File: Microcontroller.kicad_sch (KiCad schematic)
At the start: 36 parts, among them IC201 ESP32-S3-WROOM-1-N4, SW201 NRST, SW202 USER, SW203 USER, SW204 USER, U201 STM32F405RGTx, Y201 16MHz|9p|10ppm

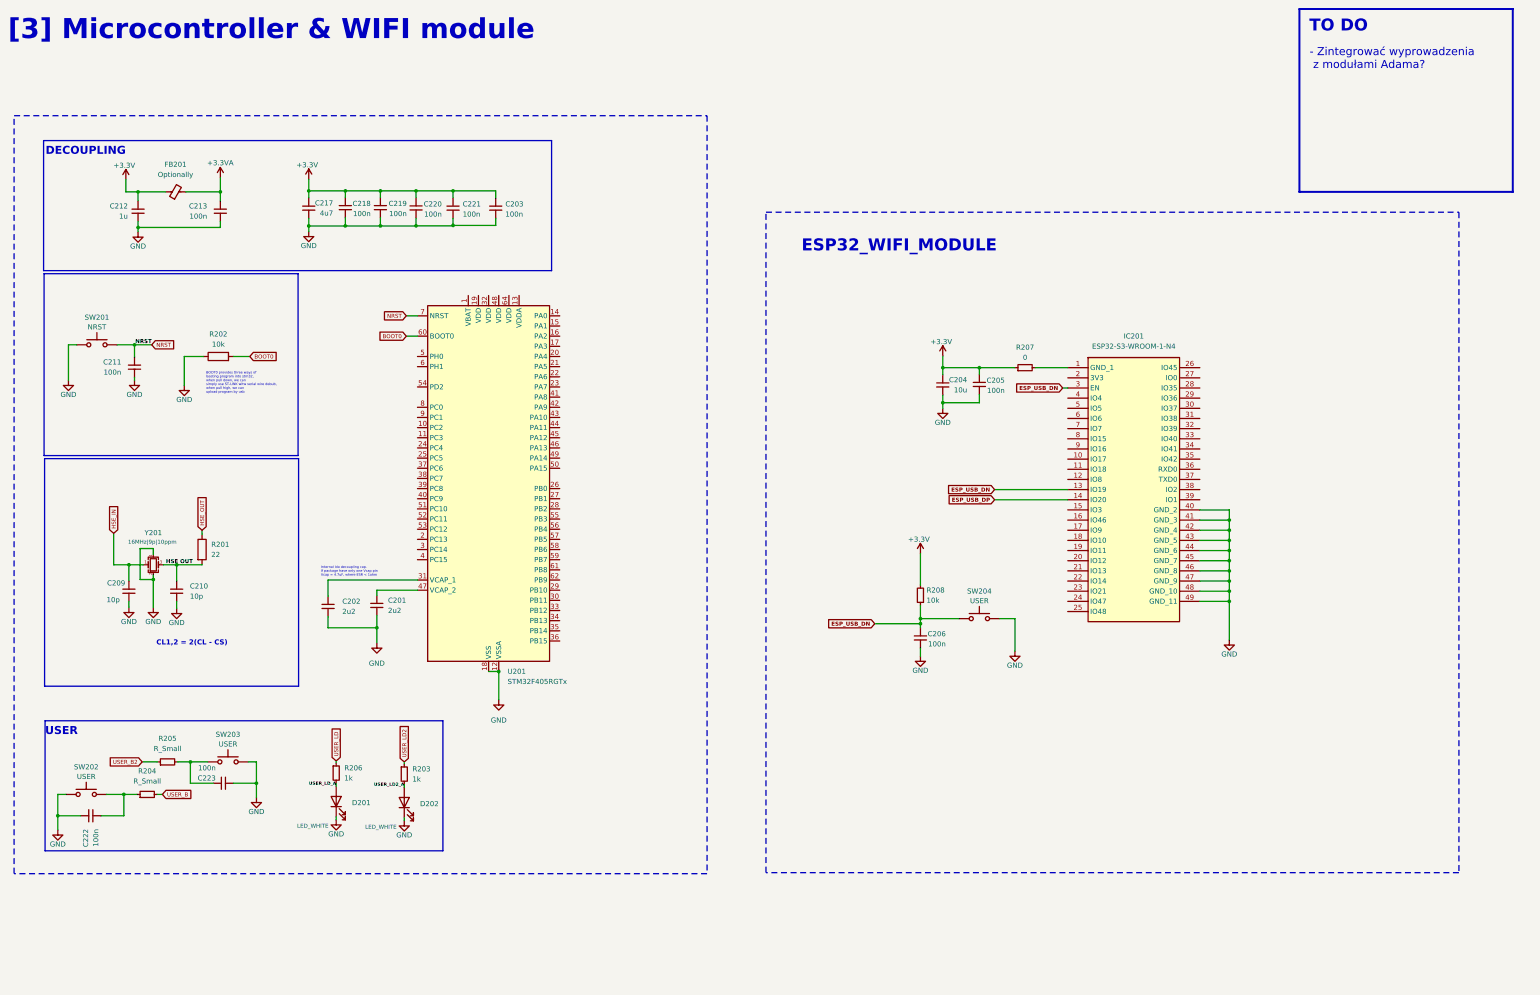
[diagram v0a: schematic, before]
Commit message: Dodaje wszystko nie chce mi sie z tym bawic
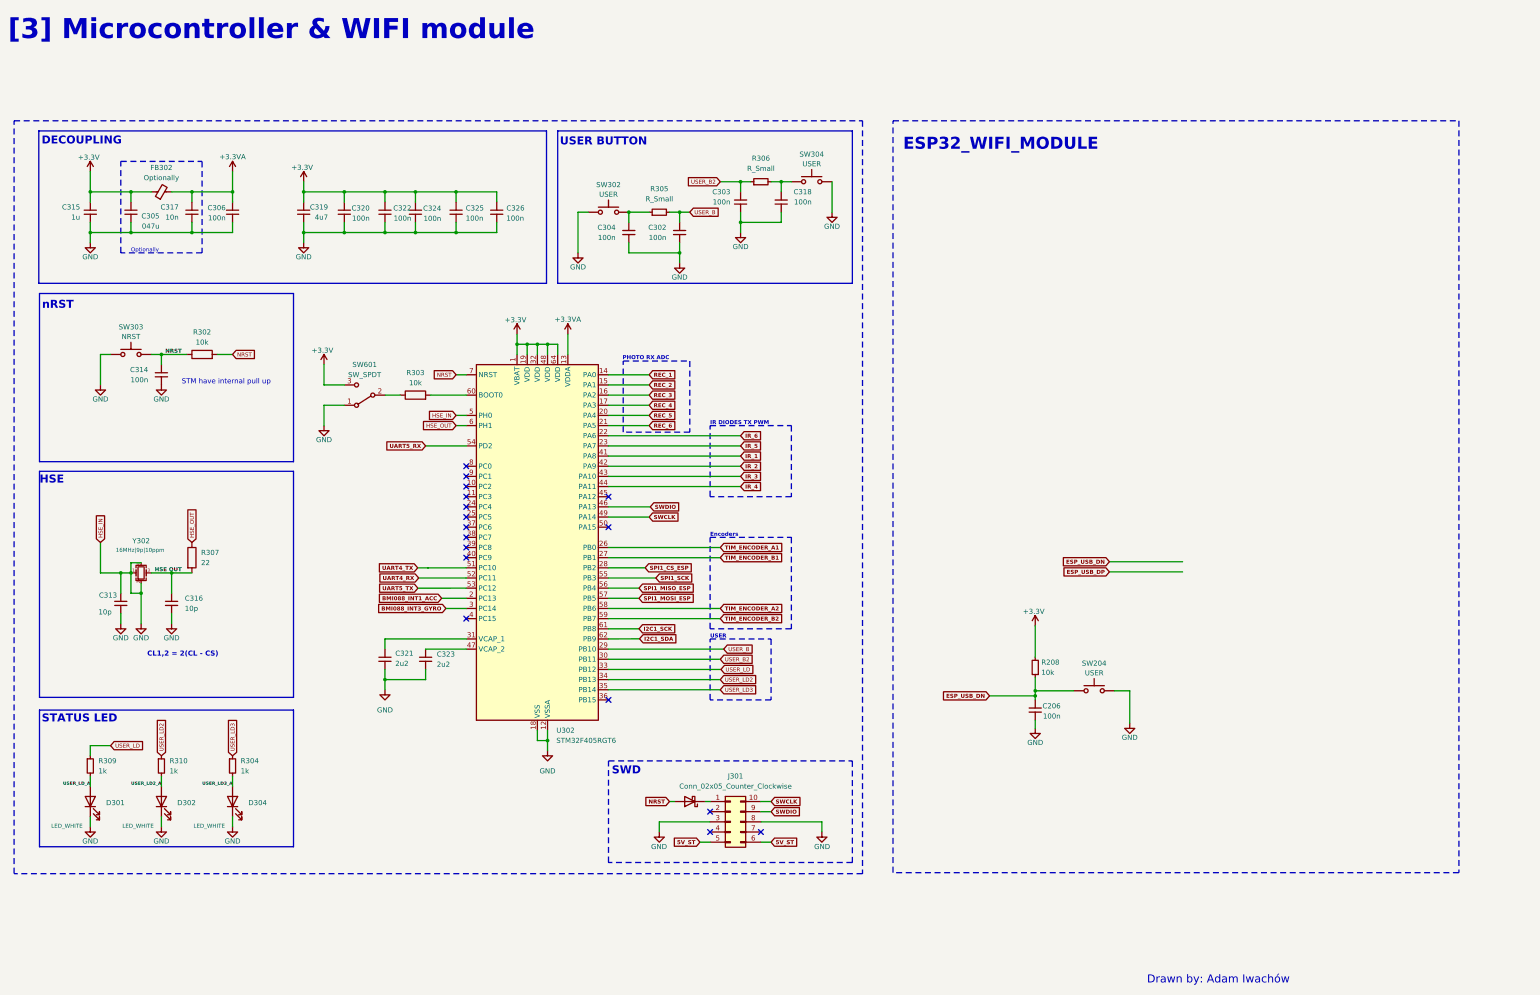
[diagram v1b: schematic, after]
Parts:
- removed C201, C202: 2u2, symbol Device:C_Small
- removed C203, C205, C211, C213, C218, C219, C220, C221, C222, C223: 100n, Capacitor_SMD:C_0402_1005Metric, symbol Device:C_Small
- removed C204: 10u, Capacitor_SMD:C_0603_1608Metric, symbol Device:C_Small
- removed C209, C210: 10p, Capacitor_SMD:C_0402_1005Metric, symbol Device:C_Small
- removed C212: 1u, Capacitor_SMD:C_0603_1608Metric, symbol Device:C_Small
- removed C217: 4u7, Capacitor_SMD:C_0603_1608Metric, symbol Device:C_Small
- removed D201, D202: LED_WHITE, Diode_SMD:D_0603_1608Metric, symbol Device:LED
- removed FB201: Optionally, symbol Device:FerriteBead_Small
- removed IC201: ESP32-S3-WROOM-1-N4, ESP32S3WROOM1N4, symbol SamacSys_Parts:ESP32-S3-WROOM-1-N4
- removed R201: 22, Resistor_SMD:R_0402_1005Metric, symbol Device:R
- removed R202: 10k, Resistor_SMD:R_0402_1005Metric, symbol Device:R
- removed R203, R206: 1k, Resistor_SMD:R_0603_1608Metric, symbol Device:R_Small
- removed R204, R205: R_Small, symbol Device:R_Small
- removed R207: 0, symbol Device:R_Small
- removed SW201: NRST, Button_Switch_SMD:SW_Push_1P1T_NO_6x6mm_H9.5mm, symbol Switch:SW_MEC_5G
- removed SW202, SW203: USER, Button_Switch_SMD:SW_Push_1P1T_NO_6x6mm_H9.5mm, symbol Switch:SW_MEC_5G
- removed U201: STM32F405RGTx, Package_QFP:LQFP-64_10x10mm_P0.5mm, symbol MCU_ST_STM32F4:STM32F405RGTx
- removed Y201: 16MHz|9p|10ppm, Crystal:Crystal_SMD_3225-4Pin_3.2x2.5mm, symbol Device:Crystal_GND24_Small
- added C302, C303, C304, C306, C314, C318, C320, C322, C324, C325, C326: 100n, Capacitor_SMD:C_0603_1608Metric, symbol Device:C_Small
- added C305: 047u, Capacitor_SMD:C_0603_1608Metric, symbol Device:C_Small
- added C313, C316: 10p, Capacitor_SMD:C_0603_1608Metric, symbol Device:C_Small
- added C315: 1u, Capacitor_SMD:C_0603_1608Metric, symbol Device:C_Small
- added C317: 10n, Capacitor_SMD:C_0603_1608Metric, symbol Device:C_Small
- added C319: 4u7, Capacitor_SMD:C_0603_1608Metric, symbol Device:C_Small
- added C321, C323: 2u2, Capacitor_SMD:C_0603_1608Metric, symbol Device:C_Small
- added D301, D302, D304: LED_WHITE, Diode_SMD:D_0603_1608Metric, symbol Device:LED
- added D602: D_Schottky, Adam_lib:D_SOD-123FL, symbol Device:D_Schottky
- added FB302: Optionally, Inductor_SMD:L_0603_1608Metric, symbol Device:FerriteBead_Small
- added J301: Conn_02x05_Counter_Clockwise, symbol Connector_Generic:Conn_02x05_Counter_Clockwise
- added R302, R303: 10k, Resistor_SMD:R_0603_1608Metric, symbol Device:R
- added R304, R309, R310: 1k, Resistor_SMD:R_0603_1608Metric, symbol Device:R_Small
- added R305, R306: R_Small, Resistor_SMD:R_0603_1608Metric, symbol Device:R_Small
- added R307: 22, Resistor_SMD:R_0603_1608Metric, symbol Device:R
- added SW302, SW304: USER, Button_Switch_SMD:SW_Push_1P1T_NO_6x6mm_H9.5mm, symbol Switch:SW_MEC_5G
- added SW303: NRST, Button_Switch_SMD:SW_Push_1P1T_NO_6x6mm_H9.5mm, symbol Switch:SW_MEC_5G
- added SW601: SW_SPDT, symbol Switch:SW_SPDT
- added U302: STM32F405RGT6, Package_QFP:LQFP-64_10x10mm_P0.5mm, symbol MCU_ST_STM32F4:STM32F405RGTx
- added Y302: 16MHz|9p|10ppm, Crystal:Crystal_SMD_3225-4Pin_3.2x2.5mm, symbol Device:Crystal_GND24_Small
- C206: footprint Capacitor_SMD:C_0402_1005Metric -> Capacitor_SMD:C_0603_1608Metric
- R208: footprint (none) -> Resistor_SMD:R_0603_1608Metric
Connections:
- net +3.3V: now also C305.1, C315.1, C319.1, C320.1, C322.1, C324.1, C325.1, C326.1, FB302.1, SW601.3 (C), U302.1 (VBAT), U302.19 (VDD), U302.32 (VDD), U302.48 (VDD), U302.64 (VDD)
- net +3.3VA: now also C306.1, C317.1, FB302.2, U302.13 (VDDA)
- net GND: now also C302.2, C303.1, C304.2, C305.2, C306.2, C313.1, C313.2, C314.2, C315.2, C316.2, C317.2, C318.1, C319.2, C320.2, C321.2, C322.2, C323.2, C324.2, C325.2, C326.2, D301.1 (K), D302.1 (K), D304.1 (K), J301.3 (Pin_3), J301.8 (Pin_8), SW302.3 (B), SW302.4 (B), SW303.3 (B), SW303.4 (B), SW304.3 (B), SW304.4 (B), SW601.1 (A), U302.12 (VSSA), U302.18 (VSS), U302.5 (PH0), U302.63 (VSS), Y302.1, Y302.2, Y302.4
- net HSE OUT: now also C316.1, R307.2, Y302.3
- net HSE_OUT: now also R307.1, U302.6 (PH1)
- net NRST: now also C314.1, D602.2 (A), R302.1, R302.2, SW303.1 (A), SW303.2 (A), U302.7 (NRST)
- net USER_B: now also C302.1, R305.2, U302.29 (PB10)
- net USER_B2: now also C303.2, R306.1, U302.30 (PB11)
- net USER_LD: now also R309.1, U302.33 (PB12)
- net USER_LD2: now also R310.1, U302.34 (PB13)
- net USER_LD2_A: now also D302.2 (A), R310.2
- net USER_LD_A: now also D301.2 (A), R309.2
- new net: C318.2, R306.2, SW304.1 (A), SW304.2 (A)
- new net: C304.1, R305.1, SW302.1 (A), SW302.2 (A)
- new net: D602.1 (K), J301.1 (Pin_1)
- new net: C321.1, U302.31 (VCAP_1)
- new net: C323.1, U302.47 (VCAP_2)
- new net: R303.2, U302.60 (BOOT0)
- new net: R303.1, SW601.2 (B)
- new net 5V_ST: J301.5 (Pin_5), J301.6 (Pin_6)
- new net BMI088_INT1_ACC: U302.2 (PC13)
- new net BMI088_INT3_GYRO: U302.3 (PC14)
- new net I2C1_SCK: U302.61 (PB8)
- new net I2C1_SDA: U302.62 (PB9)
- new net IR_1: U302.41 (PA8)
- new net IR_2: U302.42 (PA9)
- new net IR_3: U302.43 (PA10)
- new net IR_4: U302.44 (PA11)
- new net IR_5: U302.23 (PA7)
- new net IR_6: U302.22 (PA6)
- new net REC_1: U302.14 (PA0)
- new net REC_2: U302.15 (PA1)
- new net REC_3: U302.16 (PA2)
- new net REC_4: U302.17 (PA3)
- new net REC_5: U302.20 (PA4)
- new net REC_6: U302.21 (PA5)
- new net SPI1_CS_ESP: U302.28 (PB2)
- new net SPI1_MISO_ESP: U302.56 (PB4)
- new net SPI1_MOSI_ESP: U302.57 (PB5)
- new net SPI1_SCK: U302.55 (PB3)
- new net SWCLK: J301.10 (Pin_10), U302.49 (PA14)
- new net SWDIO: J301.9 (Pin_9), U302.46 (PA13)
- new net TIM_ENCODER_A1: U302.26 (PB0)
- new net TIM_ENCODER_A2: U302.58 (PB6)
- new net TIM_ENCODER_B1: U302.27 (PB1)
- new net TIM_ENCODER_B2: U302.59 (PB7)
- new net UART4_RX: U302.52 (PC11)
- new net UART4_TX: U302.51 (PC10)
- new net UART5_RX: U302.54 (PD2)
- new net UART5_TX: U302.53 (PC12)
- new net USER_LD3: R304.1, U302.35 (PB14)
- new net USER_LD3_A: D304.2 (A), R304.2
- no-connect marks 0 -> 17
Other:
- note added: "Drawn by: Adam Iwachów"
- note added: "Encoders"
- note added: "HSE"
- note added: "IR DIODES TX PWM"
- note added: "Optionally"
- note added: "PHOTO RX ADC"
- note added: "STATUS LED"
- note added: "STM have internal pull up"
- note added: "SWD"
- note added: "USER BUTTON"
- note added: "nRST"
- note removed: "- Zintegrować wyprowadzenia z modułami Adama?"
- note removed: "BOOT0 provides three ways of booting program into stm32, when pull down, we can simply use ST-LINK witw serial wire debub, when pull high, we can upload program by usb"
- note removed: "Internal ldo decoupling cap. If package have only one Vcap pin Vcap = 4.7uF, where ESR < 1ohm"
- note removed: "TO DO"
- moved on the sheet: C206, R208, SW204

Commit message: footprinty
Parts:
- J301: footprint (none) -> Connector_PinHeader_2.54mm:PinHeader_2x05_P2.54mm_Vertical
- SW601: footprint (none) -> Button_Switch_THT:SW_PUSH_1P1T_6x3.5mm_H4.3_APEM_MJTP1243
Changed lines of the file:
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@@
       (effects (font (size 1.27 1.27)))
     )
-    (property "Footprint" "" (at 198.12 220.98 0)
+    (property "Footprint" "Connector_PinHeader_2.54mm:PinHeader_2x05_P2.54mm_Vertical" (at 198.12 220.98 0)
       (effects (font (size 1.27 1.27)) hide)
     )
@@
       (effects (font (size 1.27 1.27)))
     )
-    (property "Footprint" "" (at 106.68 114.3 0)
-      (effects (font (size 1.27 1.27)) hide)
-    )
+    (property "Footprint" "Button_Switch_THT:SW_PUSH_1P1T_6x3.5mm_H4.3_APEM_MJTP1243" (at 106.68 114.3 0)
+      (effects (font (size 1.27 1.27)) hide)
+    )
